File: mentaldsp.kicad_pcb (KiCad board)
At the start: 2 copper layers, 125 x 35 mm, 30 parts, among them J1 Conn_PWRJack_2x5.5mm_CUIDevic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, J5 NEMA Conn, J7 NEMA Conn, J8 NEMA Conn, U6 ESP32-S3-SUPERMINI, U7 TMC2209_N0, U8 TMC2209_N2, U9 TMC2209_N1

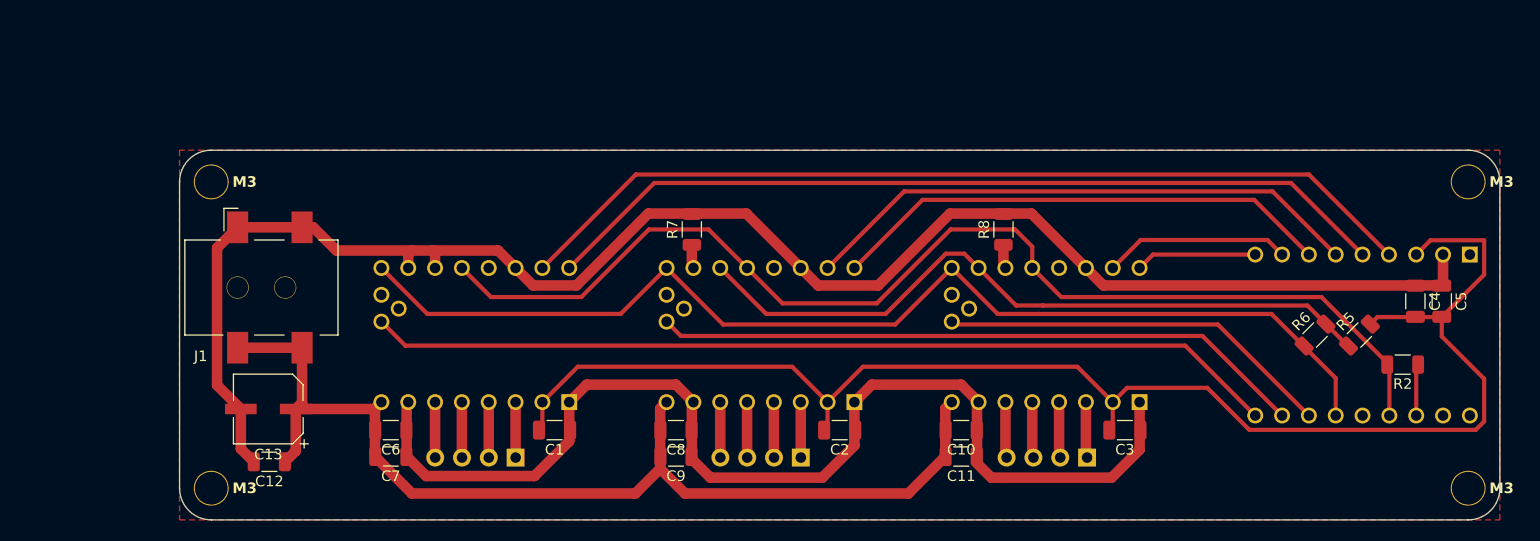
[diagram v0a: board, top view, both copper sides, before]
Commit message: housekeeping
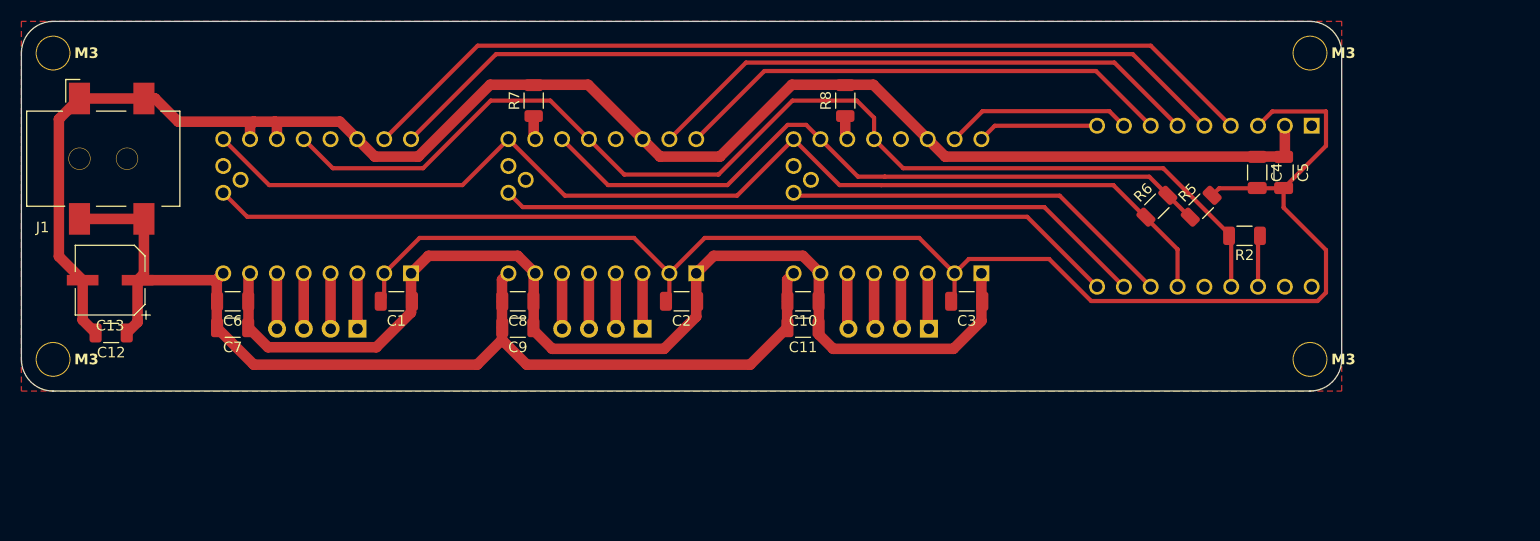
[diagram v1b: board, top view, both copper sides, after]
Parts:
- moved R2 19.3 mm to (200.8, 108.1)
- moved C13 19.3 mm to (93.4, 112.3)
- moved C1 19.3 mm to (120.5, 114.3)
- moved C10 19.3 mm to (159.0, 114.3)
- moved C11 19.3 mm to (159.0, 116.8)
- moved C12 19.3 mm to (93.5, 117.3)
- moved C2 19.3 mm to (147.5, 114.3)
- moved C3 19.3 mm to (174.5, 114.3)
- moved C4 19.3 mm to (202.0, 102.1)
- moved C5 19.3 mm to (204.5, 102.1)
- moved C6 19.3 mm to (105.0, 114.3)
- moved C7 19.3 mm to (105.0, 116.8)
- moved C8 19.3 mm to (132.0, 114.3)
- moved C9 19.3 mm to (132.0, 116.8)
- moved H1 19.3 mm to (207.0, 119.8)
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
